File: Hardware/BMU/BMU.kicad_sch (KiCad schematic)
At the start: 6 parts, among them J1 IN/GND, J2 HIGH SIDE, J3 I2C, J4 LOW SIDE, J5 SHUNT, J7 CAN

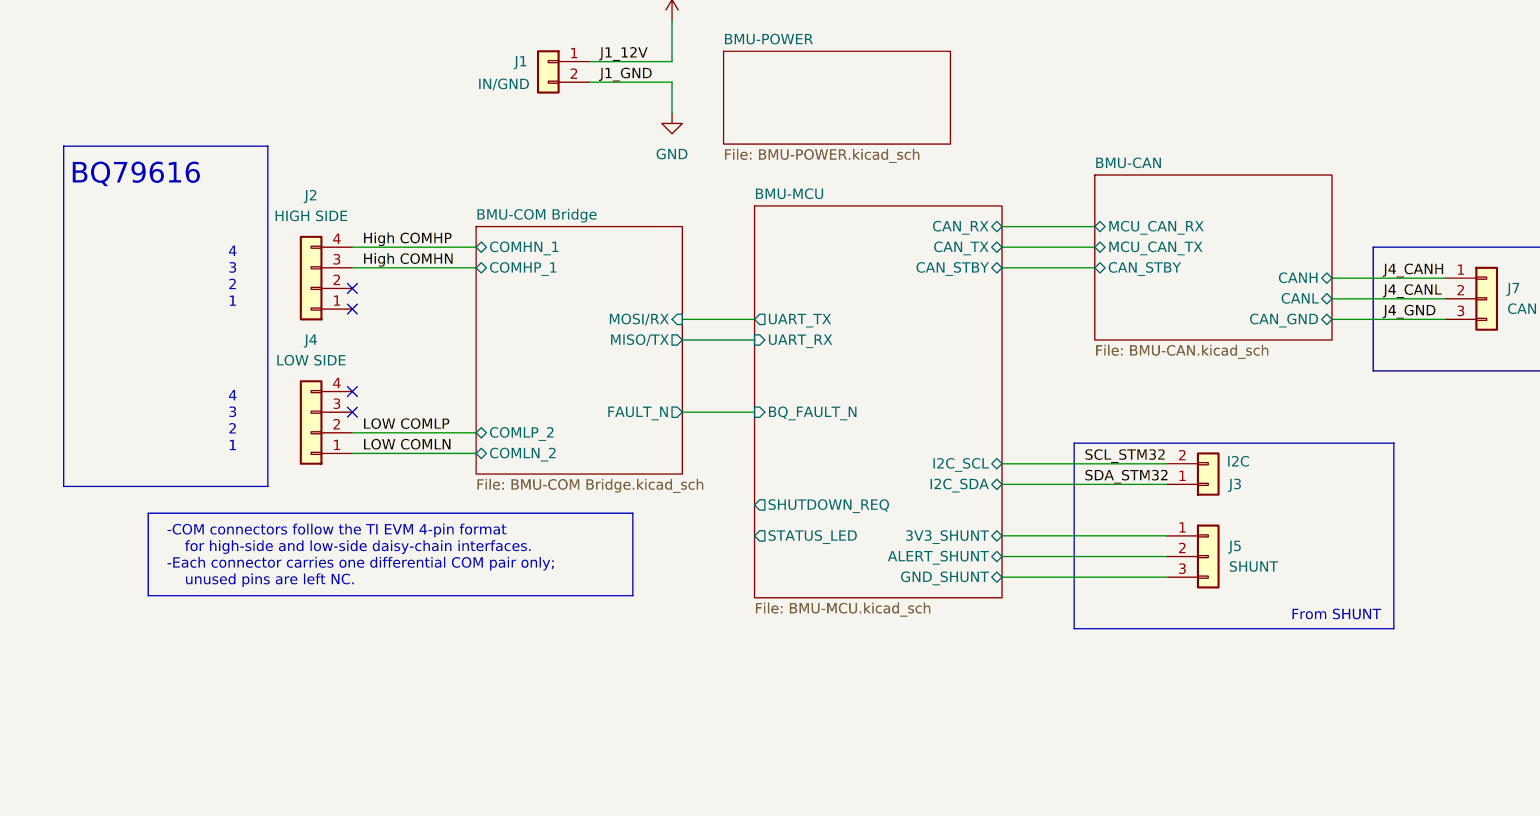
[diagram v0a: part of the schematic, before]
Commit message: layout
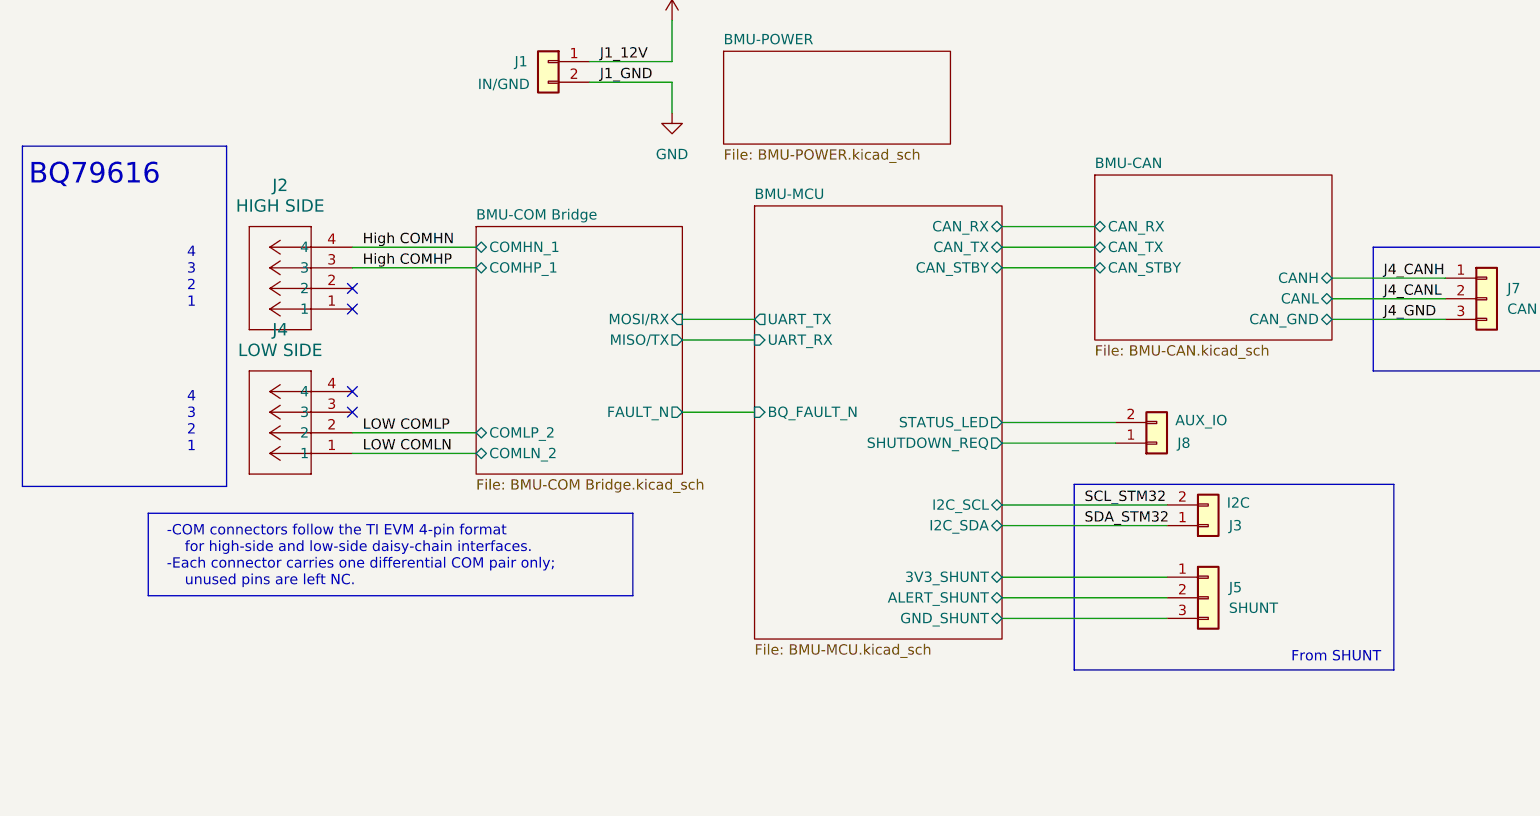
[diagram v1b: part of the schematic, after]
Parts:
- removed J2: HIGH SIDE, Connector_PinHeader_2.54mm:PinHeader_1x04_P2.54mm_Vertical, symbol Connector_Generic:Conn_01x04
- removed J4: LOW SIDE, Connector_PinHeader_2.54mm:PinHeader_1x04_P2.54mm_Vertical, symbol Connector_Generic:Conn_01x04
- added J2: HIGH SIDE, CONN_70551-xxxx_04_MOL, symbol 70551-0038:705510038
- added J4: LOW SIDE, CONN_70551-xxxx_04_MOL, symbol 70551-0038:705510038
- added J8: AUX_IO, Connector_PinHeader_2.54mm:PinHeader_1x02_P2.54mm_Vertical, symbol Connector_Generic:Conn_01x02
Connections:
- net BMU-MCU/SHUTDOWN_REQ: now also J8.1 (Pin_1)
- net BMU-MCU/STATUS_LED: now also J8.2 (Pin_2)
- net High COMHN: now also J2.4
- net High COMHP: now also J2.3
- net LOW COMLN: now also J4.1
- net LOW COMLP: now also J4.2
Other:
- sheet BMU-CAN ports: added CAN_RX, CAN_TX; removed MCU_CAN_RX, MCU_CAN_TX
- moved on the sheet: J3, J5
